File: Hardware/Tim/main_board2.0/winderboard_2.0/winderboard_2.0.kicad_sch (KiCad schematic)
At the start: 21 parts, among them J1 Conn_01x03_Socket, J10 Conn_01x04_Socket, J11 Conn_01x06_Socket, J2 Conn_01x03_Socket, J3 Conn_01x03_Socket, J4 Conn_01x03_Socket, J5 Conn_01x05_Socket, J6 Conn_01x05_Socket, J7 Conn_01x05_Socket, J8 Conn_01x02_Socket, J9 Conn_01x02_Socket, U1 DEV-16771, U2 MS5607-02BA, U3 MAX-M10S, U4 TMP100

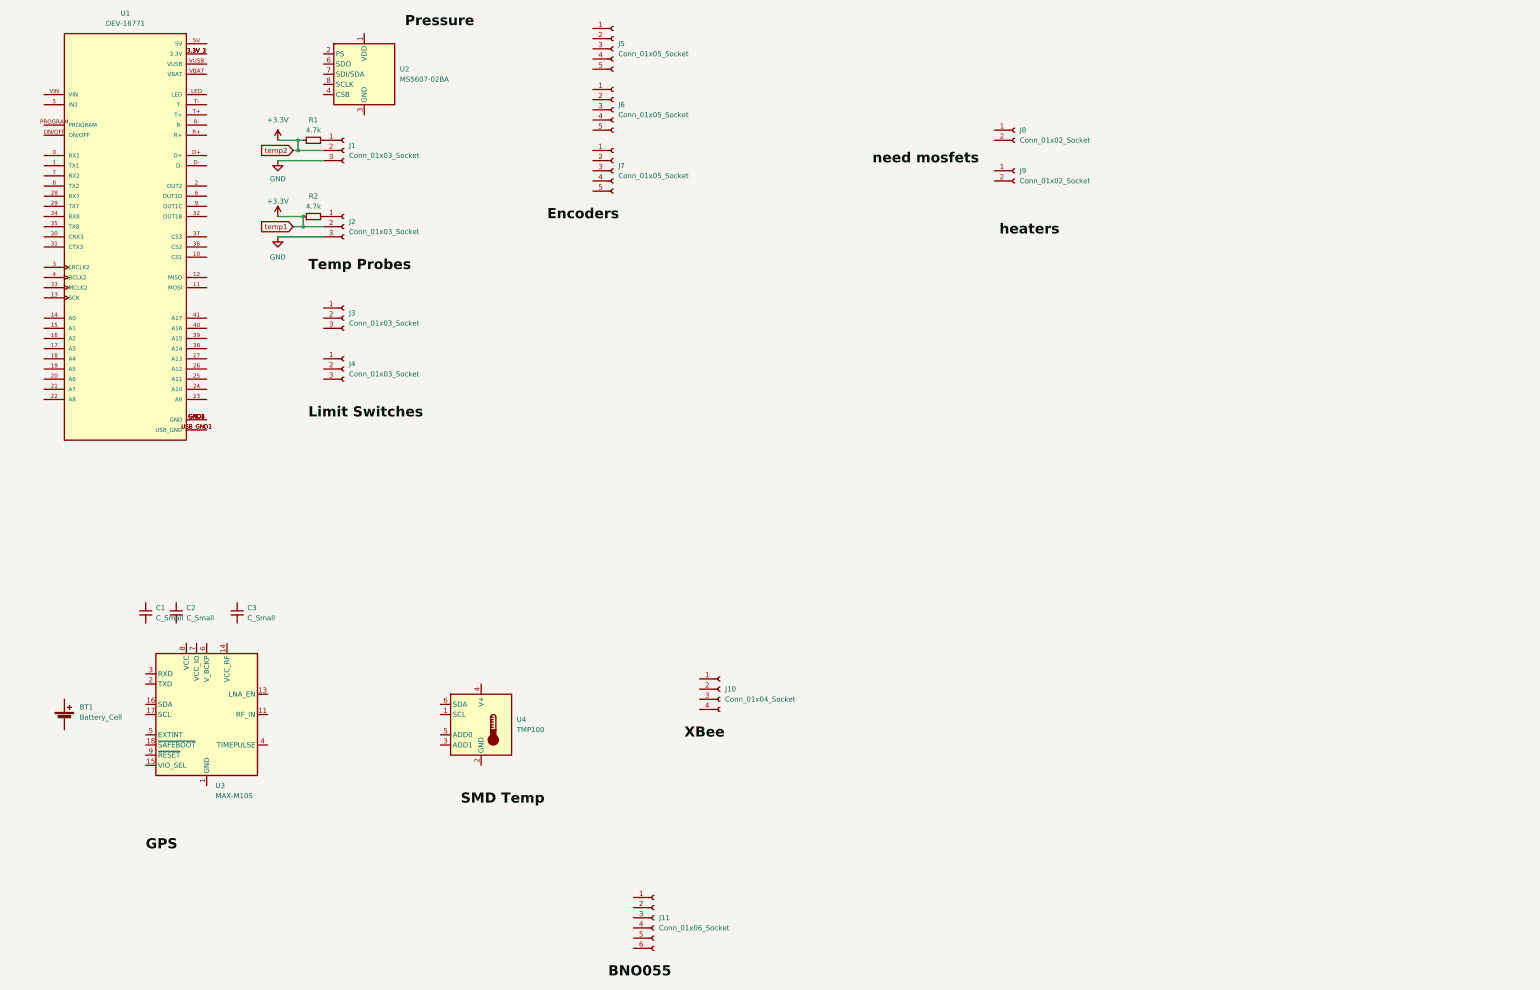
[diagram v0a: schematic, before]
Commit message: latest board
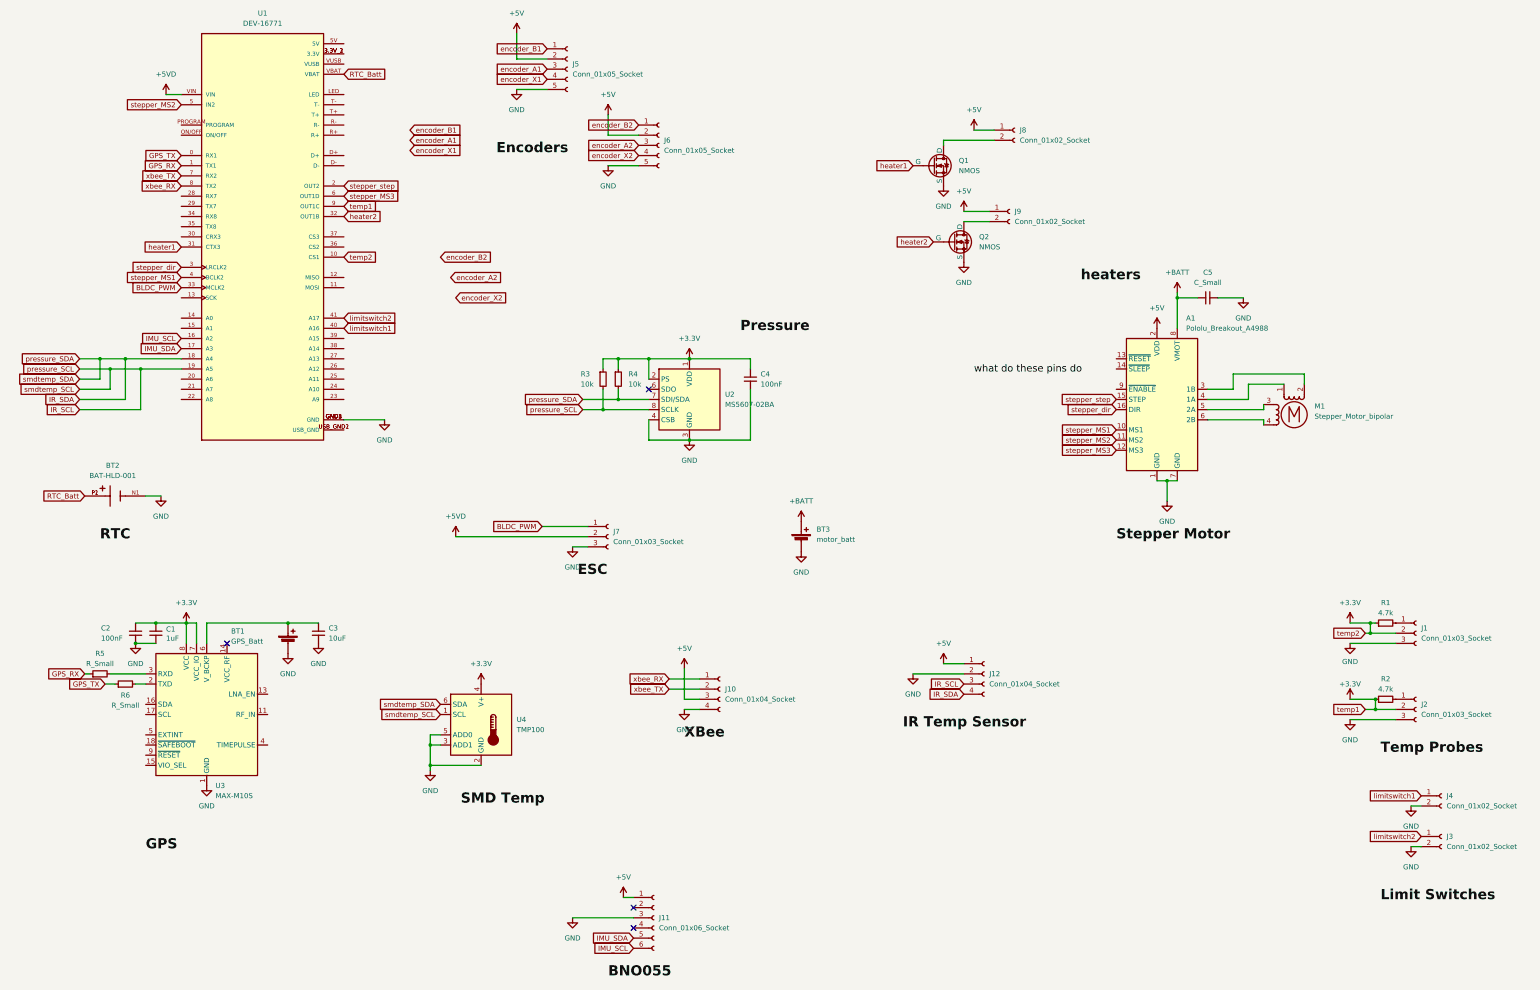
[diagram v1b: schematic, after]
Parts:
- removed J3, J4: Conn_01x03_Socket, symbol Connector:Conn_01x03_Socket
- removed J7: Conn_01x05_Socket, symbol Connector:Conn_01x05_Socket
- added A1: Pololu_Breakout_A4988, Module:Pololu_Breakout-16_15.2x20.3mm, symbol Driver_Motor:Pololu_Breakout_A4988
- added BT2: BAT-HLD-001, BAT-HLD-001:BAT_BAT-HLD-001, symbol BAT-HLD-001:BAT-HLD-001
- added BT3: motor_batt, symbol Device:Battery_Cell
- added C4: 100nF, symbol Device:C_Small
- added C5: C_Small, symbol Device:C_Small
- added J12: Conn_01x04_Socket, symbol Connector:Conn_01x04_Socket
- added J3, J4: Conn_01x02_Socket, symbol Connector:Conn_01x02_Socket
- added J7: Conn_01x03_Socket, symbol Connector:Conn_01x03_Socket
- added M1: Stepper_Motor_bipolar, symbol Motor:Stepper_Motor_bipolar
- added Q1, Q2: NMOS, Package_TO_SOT_SMD:SOT-23-3, symbol Simulation_SPICE:NMOS
- added R3, R4: 10k, symbol Device:R_Small
- added R5, R6: R_Small, symbol Device:R_Small
- BT1: value Battery_Cell -> GPS_Batt
- C1: value C_Small -> 1uF
- C2: value C_Small -> 100nF
- C3: value C_Small -> 10uF
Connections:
- net +3.3V: now also C1.1, C2.2, U1.10 (CS1), U1.9 (OUT1C), U2.1 (VDD), U2.2 (PS), U3.7 (VCC_IO), U3.8 (VCC), U4.4 (V+), C4.1, R3.1, R4.1
- net GND: now also BT1.2 (-), C1.2, C2.1, C3.2, J10.4 (Pin_4), J11.3 (Pin_3), J5.5 (Pin_5), J6.5 (Pin_5), U1.GND1 (GND), U1.GND2 (GND), U1.GND3 (GND), U1.GND4 (GND), U1.GND5 (GND), U2.3 (GND), U2.4 (CSB), U2.5 (CSB), U3.1 (GND), U3.10 (GND), U3.12 (GND), U4.2 (GND), U4.3 (ADD1), U4.5 (ADD0), A1.1 (GND), A1.7 (GND), BT2.N1, BT3.2 (-), C4.2, C5.2, J12.2 (Pin_2), J3.2 (Pin_2), J4.2 (Pin_2), J7.3 (Pin_3), Q1.3 (S), Q2.3 (S)
- net at C3.1: now also BT1.1 (+), U3.6 (V_BCKP)
- net xbee_RX: now reaches J10.1 (Pin_1)
- net xbee_RX: now also U1.8 (TX2)
- net xbee_TX: now reaches J10.2 (Pin_2)
- net xbee_TX: now also U1.7 (RX2)
- net +5V: now reaches J10.3 (Pin_3)
- net +5V: now also J11.1 (Pin_1), J5.2 (Pin_2), J6.2 (Pin_2), J8.1 (Pin_1), J9.1 (Pin_1), A1.2 (VDD), J12.1 (Pin_1)
- net IR_SDA: now reaches U2.7 (SDI/SDA)
- net IR_SDA: now also U1.18 (A4), U4.6 (SDA), J12.4 (Pin_4), R4.2
- net IR_SCL: now reaches U2.8 (SCLK)
- net IR_SCL: now also U1.19 (A5), U4.1 (SCL), J12.3 (Pin_3), R3.2
- net encoder_B2: now reaches J6.1 (Pin_1)
- net encoder_A2: now reaches J6.3 (Pin_3)
- net encoder_X2: now reaches J6.4 (Pin_4)
- net IMU_SDA: now reaches J11.5 (Pin_5)
- net IMU_SDA: now also U1.17 (A3)
- net IMU_SCL: now reaches J11.6 (Pin_6)
- net IMU_SCL: now also U1.16 (A2)
- net at J8.2 (Pin_2): now also Q1.1 (D)
- net encoder_B1: now reaches J5.1 (Pin_1)
- net encoder_A1: now reaches J5.3 (Pin_3)
- net encoder_X1: now reaches J5.4 (Pin_4)
- net at U3.2 (TXD): now also R6.2
- net at U3.3 (RXD): now also R5.2
- net GPS_TX: now reaches U1.0 (RX1)
- net GPS_TX: now also R6.1
- net GPS_RX: now reaches U1.1 (TX1)
- net GPS_RX: now also R5.1
- net stepper_step: now reaches U1.2 (OUT2)
- net stepper_step: now also A1.15 (STEP)
- net stepper_dir: now reaches U1.3 (LRCLK2)
- net stepper_dir: now also A1.16 (DIR)
- net heater1: now reaches U1.31 (CTX3)
- net heater1: now also Q1.2 (G)
- net heater2: now reaches U1.32 (OUT1B)
- net heater2: now also Q2.2 (G)
- net BLDC_PWM: now reaches U1.33 (MCLK2)
- net BLDC_PWM: now also J7.1 (Pin_1)
- net stepper_MS1: now reaches U1.4 (BCLK2)
- net stepper_MS1: now also A1.10 (MS1)
- net limitswitch1: now reaches U1.40 (A16)
- net limitswitch1: now also J4.1 (Pin_1)
- net limitswitch2: now reaches U1.41 (A17)
- net limitswitch2: now also J3.1 (Pin_1)
- net stepper_MS2: now reaches U1.5 (IN2)
- net stepper_MS2: now also A1.11 (MS2)
- net stepper_MS3: now reaches U1.6 (OUT1D)
- net stepper_MS3: now also A1.12 (MS3)
- net RTC_Batt: now reaches U1.VBAT
- net RTC_Batt: now also BT2.P1, BT2.P2
- net +5VD: now reaches U1.VIN
- net +5VD: now also J7.2 (Pin_2)
- net at J9.2 (Pin_2): now also Q2.1 (D)
- new net: A1.4 (1A), M1.1
- new net: A1.3 (1B), M1.2 (-)
- new net: A1.5 (2A), M1.3
- new net: A1.6 (2B), M1.4
- new net +BATT: A1.8 (VMOT), BT3.1 (+), C5.1
- no-connect marks 0 -> 4
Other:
- moved on the sheet: BT1, C1, C2, C3, J1, J2, J5, J6, J9, R1, R2, U1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
